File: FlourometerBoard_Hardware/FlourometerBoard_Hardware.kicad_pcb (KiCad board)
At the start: 2 copper layers, 105.7 x 36.6 mm, 15 parts, among them J1 RJ45_LED_Shielded, U1 Teensy4.1_DEV-16771, U3 OKI

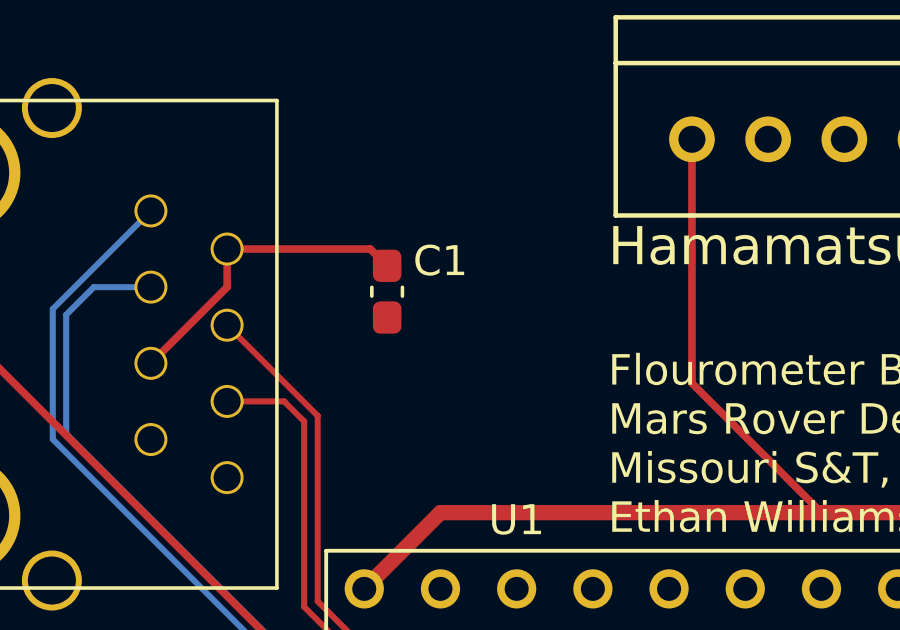
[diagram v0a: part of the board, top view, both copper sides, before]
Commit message: Final Revisions
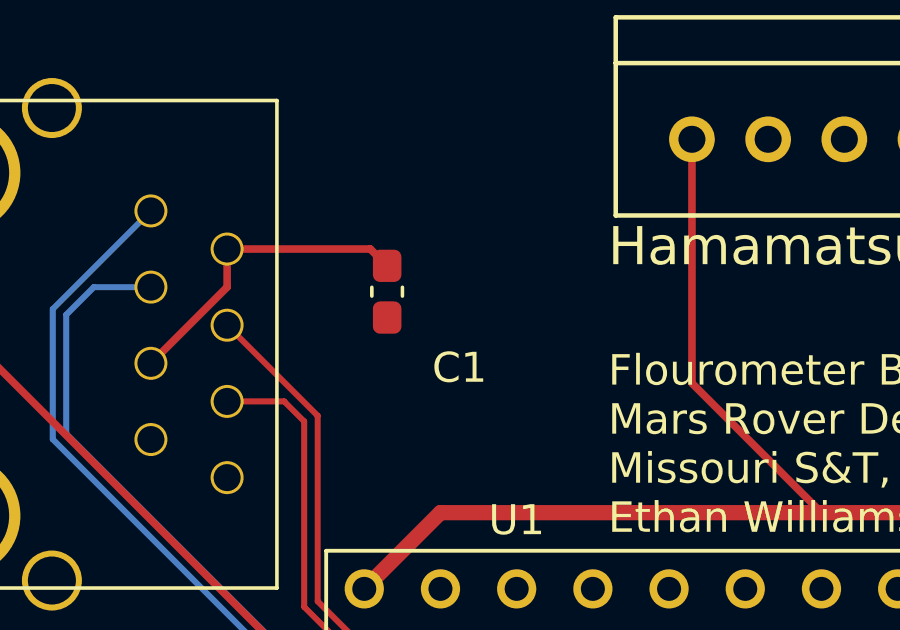
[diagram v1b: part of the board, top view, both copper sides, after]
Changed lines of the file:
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@@
     (property "ki_keywords" "cap capacitor")
     (attr smd)
-    (fp_text reference "C1" (at 1.016 1.778 180) (layer "F.SilkS")
+    (fp_text reference "C1" (at -2.54 2.413 180) (layer "F.SilkS")
         (effects (font (size 1 1) (thickness 0.15)))
     )
